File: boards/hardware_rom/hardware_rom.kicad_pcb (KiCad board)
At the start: 2 copper layers, 43.8 x 60.3 mm, 16 parts, among them J1 Conn_02x10_Top_Bottom, J2 Conn_01x02, J3 Conn_01x08, SW1 addr_high, U1 27C512

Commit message: adjust for creating gerver files
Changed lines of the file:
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@@
     (aux_axis_origin 159.385 52.705)
     (pcbplotparams
-      (layerselection 0x00010fc_ffffffff)
+      (layerselection 0x00010f0_ffffffff)
       (disableapertmacros false)
       (usegerberextensions false)
@@
       (viasonmask false)
       (mode 1)
-      (useauxorigin false)
+      (useauxorigin true)
       (hpglpennumber 1)
       (hpglpenspeed 20)
@@
       (outputformat 1)
       (mirror false)
-      (drillshape 1)
+      (drillshape 0)
       (scaleselection 1)
-      (outputdirectory "")
+      (outputdirectory "../../../release/todo_tag_here/work/hardware_rom/")
     )
   )
@@
     (fp_line (start 1 0.625) (end 1 -0.625) (layer "B.Fab") (width 0.1))
     (fp_line (start -1 -0.625) (end -1 0.625) (layer "B.Fab") (width 0.1))
-    (pad "1" smd roundrect (at -1 0) (size 1.2 1.4) (layers "B.Cu" "B.Paste" "B.Mask") (roundrect_rratio 0.208333)
+    (pad "1" smd roundrect (at -1 0) (size 1.2 1.4) (layers "B.Cu" "B.Paste" "B.Mask") (roundrect_rratio 0.2083333333)
       (net 24 "Net-(J3-Pad4)") (pintype "passive"))
-    (pad "2" smd roundrect (at 1 0) (size 1.2 1.4) (layers "B.Cu" "B.Paste" "B.Mask") (roundrect_rratio 0.208333)
+    (pad "2" smd roundrect (at 1 0) (size 1.2 1.4) (layers "B.Cu" "B.Paste" "B.Mask") (roundrect_rratio 0.2083333333)
       (net 2 "GND") (pintype "passive"))
     (model "${KICAD6_3DMODEL_DIR}/Resistor_SMD.3dshapes/R_0805_2012Metric.wrl"
@@
     (fp_line (start -1 -0.625) (end -1 0.625) (layer "B.Fab") (width 0.1))
     (fp_line (start 1 0.625) (end 1 -0.625) (layer "B.Fab") (width 0.1))
-    (pad "1" smd roundrect (at -1.0375 0 180) (size 1.175 1.45) (layers "B.Cu" "B.Paste" "B.Mask") (roundrect_rratio 0.212766)
+    (pad "1" smd roundrect (at -1.0375 0 180) (size 1.175 1.45) (layers "B.Cu" "B.Paste" "B.Mask") (roundrect_rratio 0.2127659574)
       (net 1 "VCC") (pintype "passive"))
-    (pad "2" smd roundrect (at 1.0375 0 180) (size 1.175 1.45) (layers "B.Cu" "B.Paste" "B.Mask") (roundrect_rratio 0.212766)
+    (pad "2" smd roundrect (at 1.0375 0 180) (size 1.175 1.45) (layers "B.Cu" "B.Paste" "B.Mask") (roundrect_rratio 0.2127659574)
       (net 2 "GND") (pintype "passive"))
     (model "${KICAD6_3DMODEL_DIR}/Capacitor_SMD.3dshapes/C_0805_2012Metric.wrl"
@@
     (fp_line (start 1 0.625) (end 1 -0.625) (layer "B.Fab") (width 0.1))
     (fp_line (start -1 -0.625) (end -1 0.625) (layer "B.Fab") (width 0.1))
-    (pad "1" smd roundrect (at -1 0) (size 1.2 1.4) (layers "B.Cu" "B.Paste" "B.Mask") (roundrect_rratio 0.208333)
+    (pad "1" smd roundrect (at -1 0) (size 1.2 1.4) (layers "B.Cu" "B.Paste" "B.Mask") (roundrect_rratio 0.2083333333)
       (net 28 "Net-(J3-Pad8)") (pintype "passive"))
-    (pad "2" smd roundrect (at 1 0) (size 1.2 1.4) (layers "B.Cu" "B.Paste" "B.Mask") (roundrect_rratio 0.208333)
+    (pad "2" smd roundrect (at 1 0) (size 1.2 1.4) (layers "B.Cu" "B.Paste" "B.Mask") (roundrect_rratio 0.2083333333)
       (net 2 "GND") (pintype "passive"))
     (model "${KICAD6_3DMODEL_DIR}/Resistor_SMD.3dshapes/R_0805_2012Metric.wrl"
@@
     (fp_line (start 1 -0.625) (end -1 -0.625) (layer "B.Fab") (width 0.1))
     (fp_line (start -1 -0.625) (end -1 0.625) (layer "B.Fab") (width 0.1))
-    (pad "1" smd roundrect (at -1 0) (size 1.2 1.4) (layers "B.Cu" "B.Paste" "B.Mask") (roundrect_rratio 0.208333)
+    (pad "1" smd roundrect (at -1 0) (size 1.2 1.4) (layers "B.Cu" "B.Paste" "B.Mask") (roundrect_rratio 0.2083333333)
       (net 25 "Net-(J3-Pad5)") (pintype "passive"))
-    (pad "2" smd roundrect (at 1 0) (size 1.2 1.4) (layers "B.Cu" "B.Paste" "B.Mask") (roundrect_rratio 0.208333)
+    (pad "2" smd roundrect (at 1 0) (size 1.2 1.4) (layers "B.Cu" "B.Paste" "B.Mask") (roundrect_rratio 0.2083333333)
       (net 2 "GND") (pintype "passive"))
     (model "${KICAD6_3DMODEL_DIR}/Resistor_SMD.3dshapes/R_0805_2012Metric.wrl"
@@
     (fp_line (start -1 0.625) (end 1 0.625) (layer "B.Fab") (width 0.1))
     (fp_line (start -1 -0.625) (end -1 0.625) (layer "B.Fab") (width 0.1))
-    (pad "1" smd roundrect (at -1 0) (size 1.2 1.4) (layers "B.Cu" "B.Paste" "B.Mask") (roundrect_rratio 0.208333)
+    (pad "1" smd roundrect (at -1 0) (size 1.2 1.4) (layers "B.Cu" "B.Paste" "B.Mask") (roundrect_rratio 0.2083333333)
       (net 27 "Net-(J3-Pad7)") (pintype "passive"))
-    (pad "2" smd roundrect (at 1 0) (size 1.2 1.4) (layers "B.Cu" "B.Paste" "B.Mask") (roundrect_rratio 0.208333)
+    (pad "2" smd roundrect (at 1 0) (size 1.2 1.4) (layers "B.Cu" "B.Paste" "B.Mask") (roundrect_rratio 0.2083333333)
       (net 2 "GND") (pintype "passive"))
     (model "${KICAD6_3DMODEL_DIR}/Resistor_SMD.3dshapes/R_0805_2012Metric.wrl"
@@
     (fp_line (start 1 -0.625) (end -1 -0.625) (layer "B.Fab") (width 0.1))
     (fp_line (start -1 0.625) (end 1 0.625) (layer "B.Fab") (width 0.1))
-    (pad "1" smd roundrect (at -1 0 180) (size 1.2 1.4) (layers "B.Cu" "B.Paste" "B.Mask") (roundrect_rratio 0.208333)
+    (pad "1" smd roundrect (at -1 0 180) (size 1.2 1.4) (layers "B.Cu" "B.Paste" "B.Mask") (roundrect_rratio 0.2083333333)
       (net 19 "Net-(J2-Pad1)") (pintype "passive"))
-    (pad "2" smd roundrect (at 1 0 180) (size 1.2 1.4) (layers "B.Cu" "B.Paste" "B.Mask") (roundrect_rratio 0.208333)
+    (pad "2" smd roundrect (at 1 0 180) (size 1.2 1.4) (layers "B.Cu" "B.Paste" "B.Mask") (roundrect_rratio 0.2083333333)
       (net 2 "GND") (pintype "passive"))
     (model "${KICAD6_3DMODEL_DIR}/Resistor_SMD.3dshapes/R_0805_2012Metric.wrl"
@@
     (fp_line (start 1 -0.625) (end -1 -0.625) (layer "B.Fab") (width 0.1))
     (fp_line (start 1 0.625) (end 1 -0.625) (layer "B.Fab") (width 0.1))
-    (pad "1" smd roundrect (at -1 0) (size 1.2 1.4) (layers "B.Cu" "B.Paste" "B.Mask") (roundrect_rratio 0.208333)
+    (pad "1" smd roundrect (at -1 0) (size 1.2 1.4) (layers "B.Cu" "B.Paste" "B.Mask") (roundrect_rratio 0.2083333333)
       (net 26 "Net-(J3-Pad6)") (pintype "passive"))
-    (pad "2" smd roundrect (at 1 0) (size 1.2 1.4) (layers "B.Cu" "B.Paste" "B.Mask") (roundrect_rratio 0.208333)
+    (pad "2" smd roundrect (at 1 0) (size 1.2 1.4) (layers "B.Cu" "B.Paste" "B.Mask") (roundrect_rratio 0.2083333333)
       (net 2 "GND") (pintype "passive"))
     (model "${KICAD6_3DMODEL_DIR}/Resistor_SMD.3dshapes/R_0805_2012Metric.wrl"
@@
     (fp_line (start -1 0.625) (end 1 0.625) (layer "B.Fab") (width 0.1))
     (fp_line (start 1 0.625) (end 1 -0.625) (layer "B.Fab") (width 0.1))
-    (pad "1" smd roundrect (at -1 0) (size 1.2 1.4) (layers "B.Cu" "B.Paste" "B.Mask") (roundrect_rratio 0.208333)
+    (pad "1" smd roundrect (at -1 0) (size 1.2 1.4) (layers "B.Cu" "B.Paste" "B.Mask") (roundrect_rratio 0.2083333333)
       (net 22 "Net-(J3-Pad2)") (pintype "passive"))
-    (pad "2" smd roundrect (at 1 0) (size 1.2 1.4) (layers "B.Cu" "B.Paste" "B.Mask") (roundrect_rratio 0.208333)
+    (pad "2" smd roundrect (at 1 0) (size 1.2 1.4) (layers "B.Cu" "B.Paste" "B.Mask") (roundrect_rratio 0.2083333333)
       (net 2 "GND") (pintype "passive"))
     (model "${KICAD6_3DMODEL_DIR}/Resistor_SMD.3dshapes/R_0805_2012Metric.wrl"
@@
     (fp_line (start -1 0.625) (end 1 0.625) (layer "B.Fab") (width 0.1))
     (fp_line (start 1 -0.625) (end -1 -0.625) (layer "B.Fab") (width 0.1))
-    (pad "1" smd roundrect (at -1 0) (size 1.2 1.4) (layers "B.Cu" "B.Paste" "B.Mask") (roundrect_rratio 0.208333)
+    (pad "1" smd roundrect (at -1 0) (size 1.2 1.4) (layers "B.Cu" "B.Paste" "B.Mask") (roundrect_rratio 0.2083333333)
       (net 23 "Net-(J3-Pad3)") (pintype "passive"))
-    (pad "2" smd roundrect (at 1 0) (size 1.2 1.4) (layers "B.Cu" "B.Paste" "B.Mask") (roundrect_rratio 0.208333)
+    (pad "2" smd roundrect (at 1 0) (size 1.2 1.4) (layers "B.Cu" "B.Paste" "B.Mask") (roundrect_rratio 0.2083333333)
       (net 2 "GND") (pintype "passive"))
     (model "${KICAD6_3DMODEL_DIR}/Resistor_SMD.3dshapes/R_0805_2012Metric.wrl"
@@
     (fp_line (start 1 0.625) (end 1 -0.625) (layer "B.Fab") (width 0.1))
     (fp_line (start -1 0.625) (end 1 0.625) (layer "B.Fab") (width 0.1))
-    (pad "1" smd roundrect (at -1 0) (size 1.2 1.4) (layers "B.Cu" "B.Paste" "B.Mask") (roundrect_rratio 0.208333)
+    (pad "1" smd roundrect (at -1 0) (size 1.2 1.4) (layers "B.Cu" "B.Paste" "B.Mask") (roundrect_rratio 0.2083333333)
       (net 21 "Net-(J3-Pad1)") (pintype "passive"))
-    (pad "2" smd roundrect (at 1 0) (size 1.2 1.4) (layers "B.Cu" "B.Paste" "B.Mask") (roundrect_rratio 0.208333)
+    (pad "2" smd roundrect (at 1 0) (size 1.2 1.4) (layers "B.Cu" "B.Paste" "B.Mask") (roundrect_rratio 0.2083333333)
       (net 2 "GND") (pintype "passive"))
     (model "${KICAD6_3DMODEL_DIR}/Resistor_SMD.3dshapes/R_0805_2012Metric.wrl"
@@
     (fp_line (start -1 0.625) (end 1 0.625) (layer "B.Fab") (width 0.1))
     (fp_line (start 1 -0.625) (end -1 -0.625) (layer "B.Fab") (width 0.1))
-    (pad "1" smd roundrect (at -1 0 180) (size 1.2 1.4) (layers "B.Cu" "B.Paste" "B.Mask") (roundrect_rratio 0.208333)
+    (pad "1" smd roundrect (at -1 0 180) (size 1.2 1.4) (layers "B.Cu" "B.Paste" "B.Mask") (roundrect_rratio 0.2083333333)
       (net 20 "Net-(J2-Pad2)") (pintype "passive"))
-    (pad "2" smd roundrect (at 1 0 180) (size 1.2 1.4) (layers "B.Cu" "B.Paste" "B.Mask") (roundrect_rratio 0.208333)
+    (pad "2" smd roundrect (at 1 0 180) (size 1.2 1.4) (layers "B.Cu" "B.Paste" "B.Mask") (roundrect_rratio 0.2083333333)
       (net 2 "GND") (pintype "passive"))
     (model "${KICAD6_3DMODEL_DIR}/Resistor_SMD.3dshapes/R_0805_2012Metric.wrl"

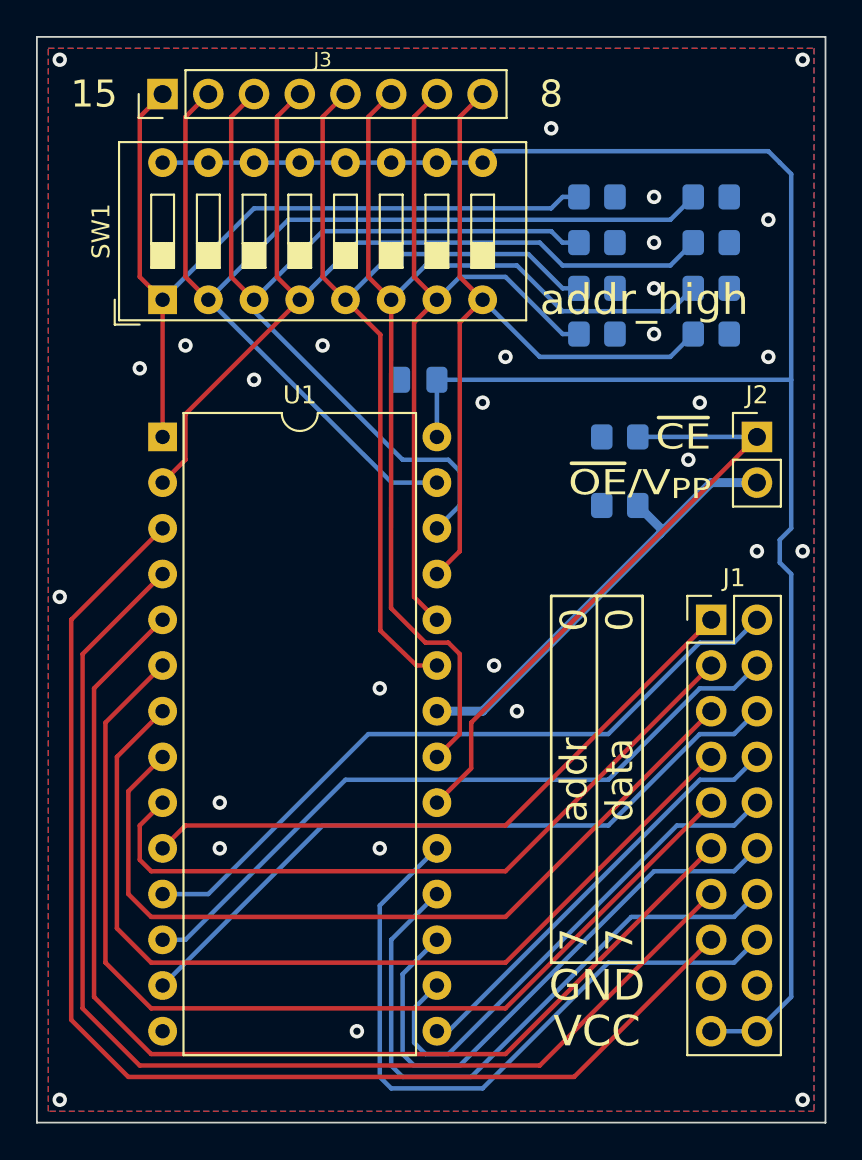
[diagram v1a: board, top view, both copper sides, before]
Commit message: unify libraries
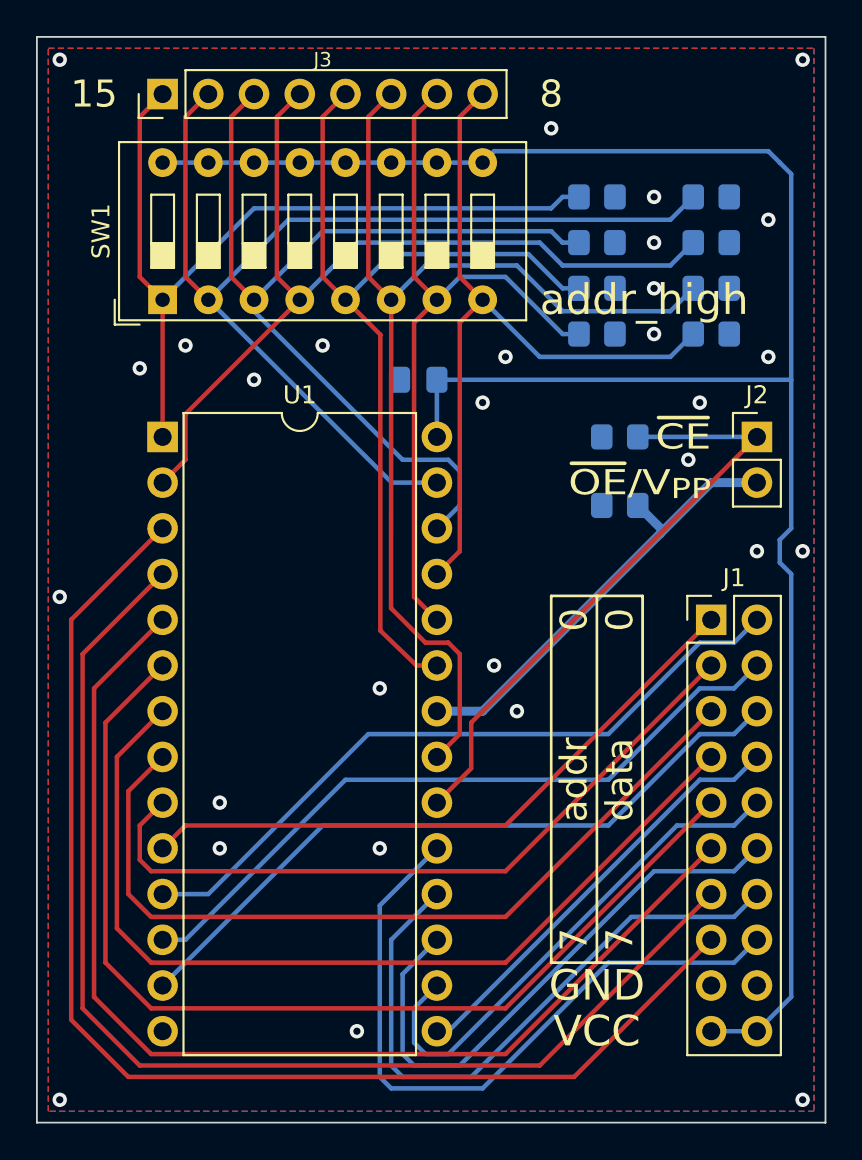
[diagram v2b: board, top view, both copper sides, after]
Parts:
- J1: footprint PrjLibrary_MainBoard:PinHeader_2x10_P2.54mm_Vertical_Top_Bottom -> ModifiedKiCadLibrary:PinHeader_2x10_P2.54mm_Vertical_Top_Bottom
- SW1: footprint Button_Switch_THT:SW_DIP_SPSTx08_Slide_9.78x22.5mm_W7.62mm_P2.54mm -> ModifiedKiCadLibrary:SW_DIP_SPSTx08_Slide_9.78x22.5mm_W7.62mm_P2.54mm_3Dfixed
- U1: footprint Package_DIP:DIP-28_W15.24mm -> ModifiedKiCadLibrary:DIP-28_W15.24mm_D1mm
